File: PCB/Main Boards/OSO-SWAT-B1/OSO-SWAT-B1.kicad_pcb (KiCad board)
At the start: 2 copper layers, 24.4 x 24.4 mm, 39 parts, among them SW0 EVP-BB1AAB000, SW1 EVP-BB1AAB000, U1 ATSAML22J18A-MUT, U3 TLV70033_WSON6, X1 32.768 kHz, 12.5 pF

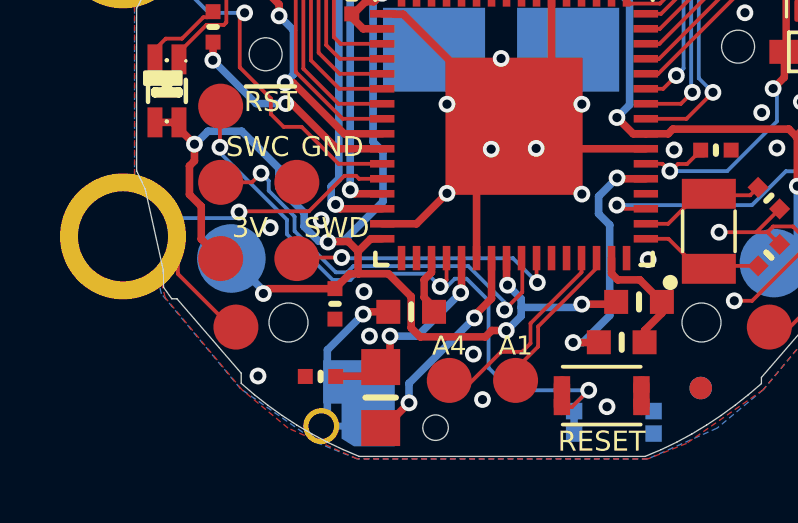
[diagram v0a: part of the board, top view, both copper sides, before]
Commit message: nudged test points further apart;  testjigulated
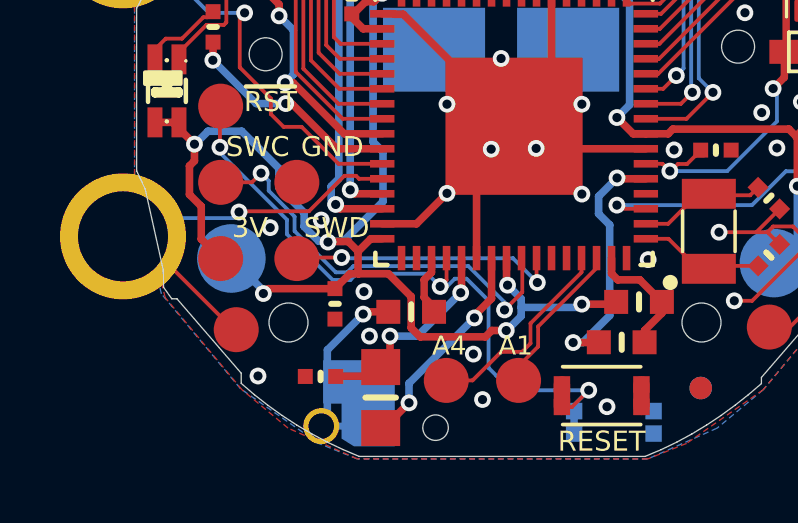
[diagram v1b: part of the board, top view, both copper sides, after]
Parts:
- moved TP6 0.10 mm to (13.1, 22.5)
- moved TP7 0.10 mm to (15.5, 22.5)
- moved TP9 0.09 mm to (6.09, 20.8)
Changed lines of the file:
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@@
 				(font
 					(size 1.27 1.27)
+					(thickness 0.15)
 				)
 			)
@@
 	(footprint "TestPoint:TestPoint_Pad_D1.5mm"
 		(layer "F.Cu")
-		(at 13.1913 22.4616 180)
+		(at 13.0913 22.4616 180)
 		(descr "SMD pad as test Point, diameter 1.5mm")
 		(tags "test point SMD pad")
@@
 				(font
 					(size 1.27 1.27)
+					(thickness 0.15)
 				)
 			)
@@
 	(footprint "TestPoint:TestPoint_Pad_D1.5mm"
 		(layer "F.Cu")
-		(at 15.4011 22.4616 180)
+		(at 15.5011 22.4616 180)
 		(descr "SMD pad as test Point, diameter 1.5mm")
 		(tags "test point SMD pad")
@@
 	(footprint "TestPoint:TestPoint_Pad_D1.5mm"
 		(layer "F.Cu")
-		(at 6.0793 20.6836 180)
+		(at 6.09 20.77 180)
 		(descr "SMD pad as test Point, diameter 1.5mm")
 		(tags "test point SMD pad")
@@
 				(font
 					(size 1.27 1.27)
+					(thickness 0.15)
 				)
 			)
@@
 	)
 	(segment
+		(start 5.76 9.73)
+		(end 5.76 10.53)
+		(width 0.127)
+		(layer "F.Cu")
+		(net "Net-(D2A-C)")
+	)
+	(segment
+		(start 5.4189 9.3889)
+		(end 5.76 9.73)
+		(width 0.127)
+		(layer "F.Cu")
+		(net "Net-(D2A-C)")
+	)
+	(segment
+		(start 5.6795 10.6105)
+		(end 5.0995 10.6105)
+		(width 0.127)
+		(layer "F.Cu")
+		(net "Net-(D2A-C)")
+	)
+	(segment
+		(start 5.4189 8.8218)
+		(end 5.4189 9.3889)
+		(width 0.127)
+		(layer "F.Cu")
+		(net "Net-(D2A-C)")
+	)
+	(segment
+		(start 5.76 10.53)
+		(end 5.6795 10.6105)
+		(width 0.127)
+		(layer "F.Cu")
+		(net "Net-(D2A-C)")
+	)
+	(segment
+		(start 5.0995 10.6105)
+		(end 4.18 11.53)
+		(width 0.127)
+		(layer "F.Cu")
+		(net "Net-(D2A-C)")
+	)
+	(segment
+		(start 4.18 11.53)
+		(end 4.18 11.7596)
+		(width 0.127)
+		(layer "F.Cu")
+		(net "Net-(D2A-C)")
+	)
+	(segment
+		(start 13.1913 22.5886)
+		(end 13.0913 22.4886)
+		(width 0.127)
+		(layer "F.Cu")
+		(net "/A4{slash}D1{slash}MISO")
+	)
+	(segment
 		(start 17.6003 18.8586)
 		(end 17.6003 18.3849)
@@
 	)
 	(segment
+		(start 15.618288 21.5096)
+		(end 15.898794 21.229094)
+		(width 0.127)
+		(layer "F.Cu")
+		(net "/A4{slash}D1{slash}MISO")
+	)
+	(segment
 		(start 15.898794 21.229094)
 		(end 15.898794 20.560106)
@@
 	)
 	(segment
-		(start 13.8403 22.5886)
-		(end 14.9193 21.5096)
+		(start 15.898794 20.560106)
+		(end 17.6003 18.8586)
 		(width 0.127)
 		(layer "F.Cu")
@@
 	)
 	(segment
-		(start 15.898794 20.560106)
-		(end 17.6003 18.8586)
+		(start 13.9673 22.4616)
+		(end 14.9193 21.5096)
 		(width 0.127)
 		(layer "F.Cu")
@@
 	)
 	(segment
-		(start 13.1913 22.5886)
-		(end 13.8403 22.5886)
+		(start 13.0913 22.4616)
+		(end 13.9673 22.4616)
 		(width 0.127)
 		(layer "F.Cu")
@@
 	)
 	(segment
-		(start 15.618288 21.5096)
-		(end 15.898794 21.229094)
+		(start 13.0913 22.4886)
+		(end 13.0913 22.4616)
 		(width 0.127)
 		(layer "F.Cu")
@@
 	)
 	(segment
+		(start 5.1308 10.3565)
+		(end 4.99429 10.3565)
+		(width 0.127)
+		(layer "F.Cu")
+		(net "Net-(D2B-C)")
+	)
+	(segment
+		(start 5.3173 10.17)
+		(end 5.1308 10.3565)
+		(width 0.127)
+		(layer "F.Cu")
+		(net "Net-(D2B-C)")
+	)
+	(segment
+		(start 3.7395 11.0691)
+		(end 3.38 11.4286)
+		(width 0.127)
+		(layer "F.Cu")
+		(net "Net-(D2B-C)")
+	)
+	(segment
+		(start 4.99429 10.3565)
+		(end 4.28169 11.0691)
+		(width 0.127)
+		(layer "F.Cu")
+		(net "Net-(D2B-C)")
+	)
+	(segment
+		(start 4.28169 11.0691)
+		(end 3.7395 11.0691)
+		(width 0.127)
+		(layer "F.Cu")
+		(net "Net-(D2B-C)")
+	)
+	(segment
+		(start 3.38 11.4286)
+		(end 3.38 11.7596)
+		(width 0.127)
+		(layer "F.Cu")
+		(net "Net-(D2B-C)")
+	)
+	(segment
 		(start 13.6003 19.5126)
 		(end 13.6003 18.3849)
@@
 	)
 	(segment
-		(start 5.9183 20.6836)
-		(end 6.0793 20.6836)
-		(width 0.127)
-		(layer "F.Cu")
-		(net "/MODE")
-	)
-	(segment
 		(start 8.513556 16.8228)
 		(end 6.2063 16.8228)
@@
 	)
 	(segment
-		(start 10.182943 15.7407)
-		(end 10.083943 15.6417)
+		(start 4.007813 18.004638)
+		(end 4.007813 18.773113)
 		(width 0.127)
 		(layer "F.Cu")
@@
 	)
 	(segment
-		(start 3.417473 17.414298)
-		(end 4.143821 18.140646)
+		(start 10.182943 15.7407)
+		(end 10.083943 15.6417)
 		(width 0.127)
 		(layer "F.Cu")
@@
 	)
 	(segment
-		(start 4.143821 18.909121)
-		(end 5.9183 20.6836)
+		(start 5.9183 20.6836)
+		(end 6.0793 20.6836)
 		(width 0.127)
 		(layer "F.Cu")
@@
 	)
 	(segment
-		(start 4.143821 18.140646)
-		(end 4.143821 18.909121)
+		(start 4.007813 18.773113)
+		(end 5.9183 20.6836)
 		(width 0.127)
 		(layer "F.Cu")
@@
 		(net "/MODE")
 	)
+	(segment
+		(start 3.417473 17.414298)
+		(end 4.007813 18.004638)
+		(width 0.127)
+		(layer "F.Cu")
+		(net "/MODE")
+	)
 	(via
 		(at 6.1809 16.8482)
@@
 		(net "/SWDIO")
 	)
-	(segment
-		(start 5.1308 10.3565)
-		(end 4.99429 10.3565)
-		(width 0.127)
-		(layer "F.Cu")
-		(net "Net-(D2B-C)")
-	)
-	(segment
-		(start 5.3173 10.17)
-		(end 5.1308 10.3565)
-		(width 0.127)
-		(layer "F.Cu")
-		(net "Net-(D2B-C)")
-	)
-	(segment
-		(start 3.7395 11.0691)
-		(end 3.38 11.4286)
-		(width 0.127)
-		(layer "F.Cu")
-		(net "Net-(D2B-C)")
-	)
-	(segment
-		(start 4.99429 10.3565)
-		(end 4.28169 11.0691)
-		(width 0.127)
-		(layer "F.Cu")
-		(net "Net-(D2B-C)")
-	)
-	(segment
-		(start 4.28169 11.0691)
-		(end 3.7395 11.0691)
-		(width 0.127)
-		(layer "F.Cu")
-		(net "Net-(D2B-C)")
-	)
-	(segment
-		(start 3.38 11.4286)
-		(end 3.38 11.7596)
-		(width 0.127)
-		(layer "F.Cu")
-		(net "Net-(D2B-C)")
-	)
-	(segment
-		(start 5.76 9.73)
-		(end 5.76 10.53)
-		(width 0.127)
-		(layer "F.Cu")
-		(net "Net-(D2A-C)")
-	)
-	(segment
-		(start 5.4189 9.3889)
-		(end 5.76 9.73)
-		(width 0.127)
-		(layer "F.Cu")
-		(net "Net-(D2A-C)")
-	)
-	(segment
-		(start 5.6795 10.6105)
-		(end 5.0995 10.6105)
-		(width 0.127)
-		(layer "F.Cu")
-		(net "Net-(D2A-C)")
-	)
-	(segment
-		(start 5.4189 8.8218)
-		(end 5.4189 9.3889)
-		(width 0.127)
-		(layer "F.Cu")
-		(net "Net-(D2A-C)")
-	)
-	(segment
-		(start 5.76 10.53)
-		(end 5.6795 10.6105)
-		(width 0.127)
-		(layer "F.Cu")
-		(net "Net-(D2A-C)")
-	)
-	(segment
-		(start 5.0995 10.6105)
-		(end 4.18 11.53)
-		(width 0.127)
-		(layer "F.Cu")
-		(net "Net-(D2A-C)")
-	)
-	(segment
-		(start 4.18 11.53)
-		(end 4.18 11.7596)
-		(width 0.127)
-		(layer "F.Cu")
-		(net "Net-(D2A-C)")
-	)
 	(zone
